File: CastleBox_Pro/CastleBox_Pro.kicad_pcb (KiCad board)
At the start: 6 copper layers, 50 x 33 mm, 86 parts, among them J1 HDMI_C_1.4, J2 USB_C_Receptacle_USB2.0_16P, J3 Conn_02x15_Odd_Even, SW1 VSEL, U1 CY7C65215-32LTXI, U2 XC6SLX9-FTG256, U3 W955K8MBYA, U4 W955K8MBYA, U5 ATtiny406-M, U6 FUSB302B10MPX, U7 AZ1117-5.0, U8 MIC5205YM5, U9 MIC5205YM5, X1 ASE-50MHz

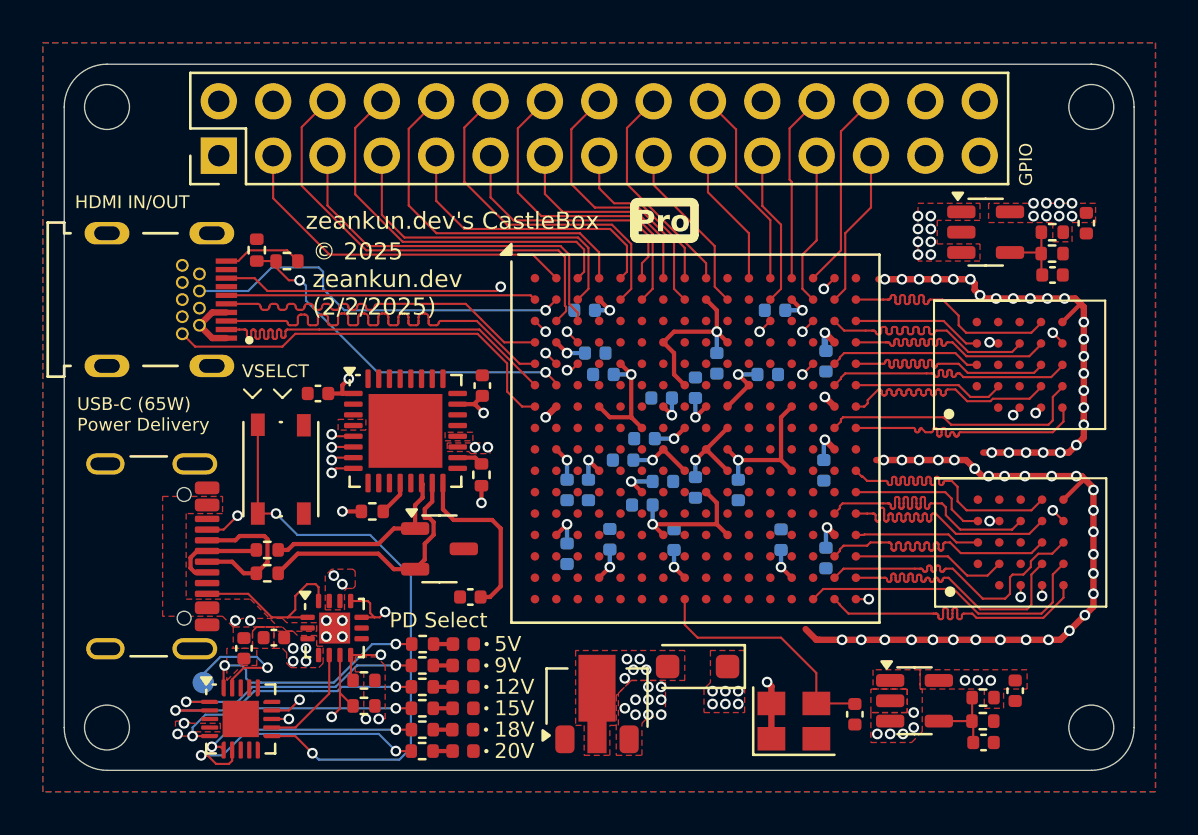
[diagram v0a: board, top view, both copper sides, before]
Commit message: sync to upstream 21/5/2025 06:52
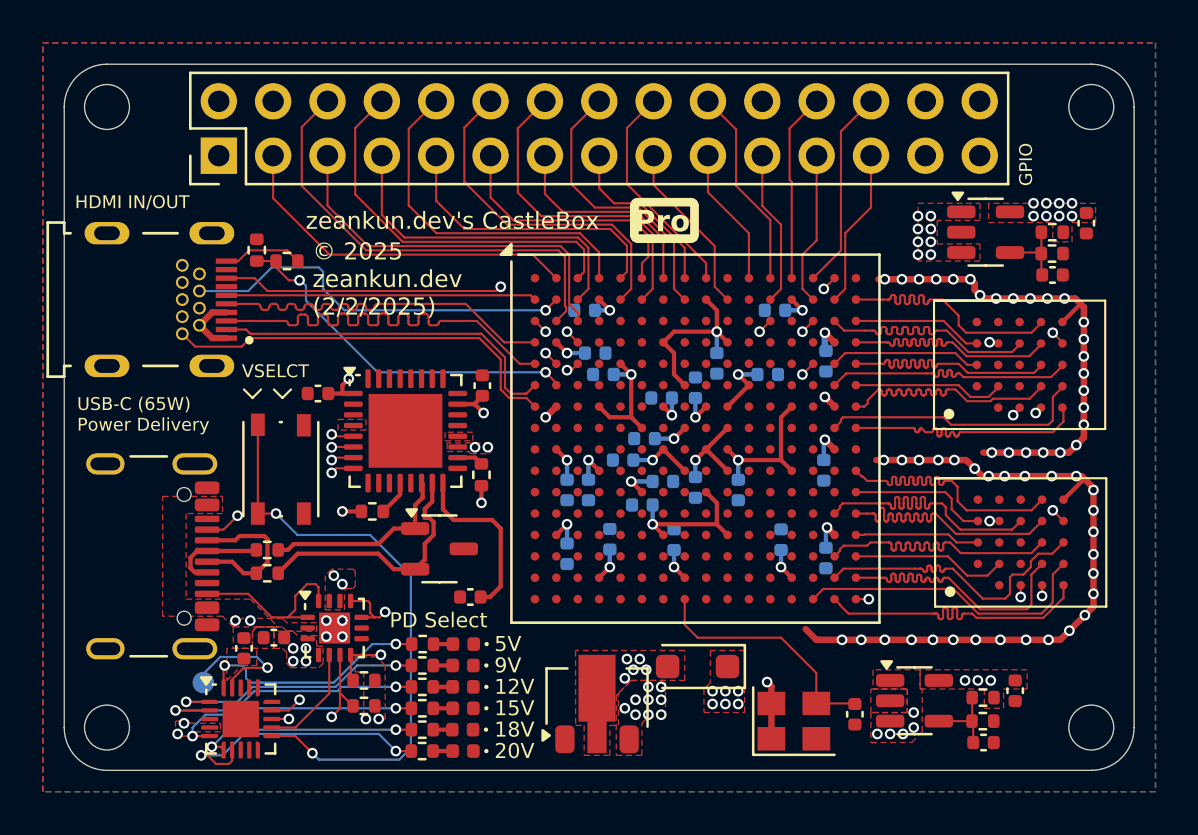
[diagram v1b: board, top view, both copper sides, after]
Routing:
- net /D2-: track 19.0 -> 16.7 mm
